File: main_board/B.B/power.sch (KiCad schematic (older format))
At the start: 30 parts, among them Q1 2N7002, Q2 2N7002, Q5 SI3447CDV, SW3 SW_DIP_x01, U62 SY8009, U63 FP6276

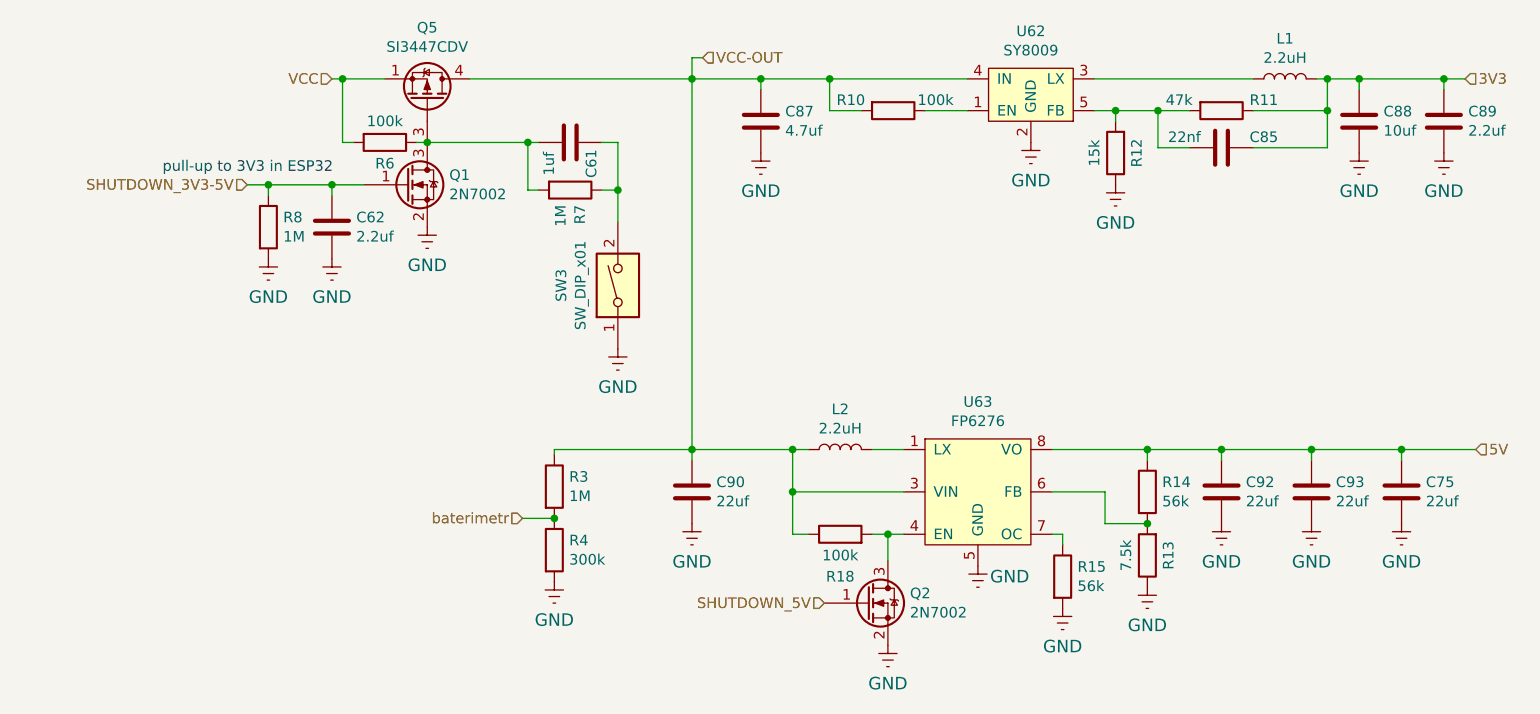
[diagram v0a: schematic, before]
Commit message: opravi_a_dodatky MPU/QMC/conn_A9G
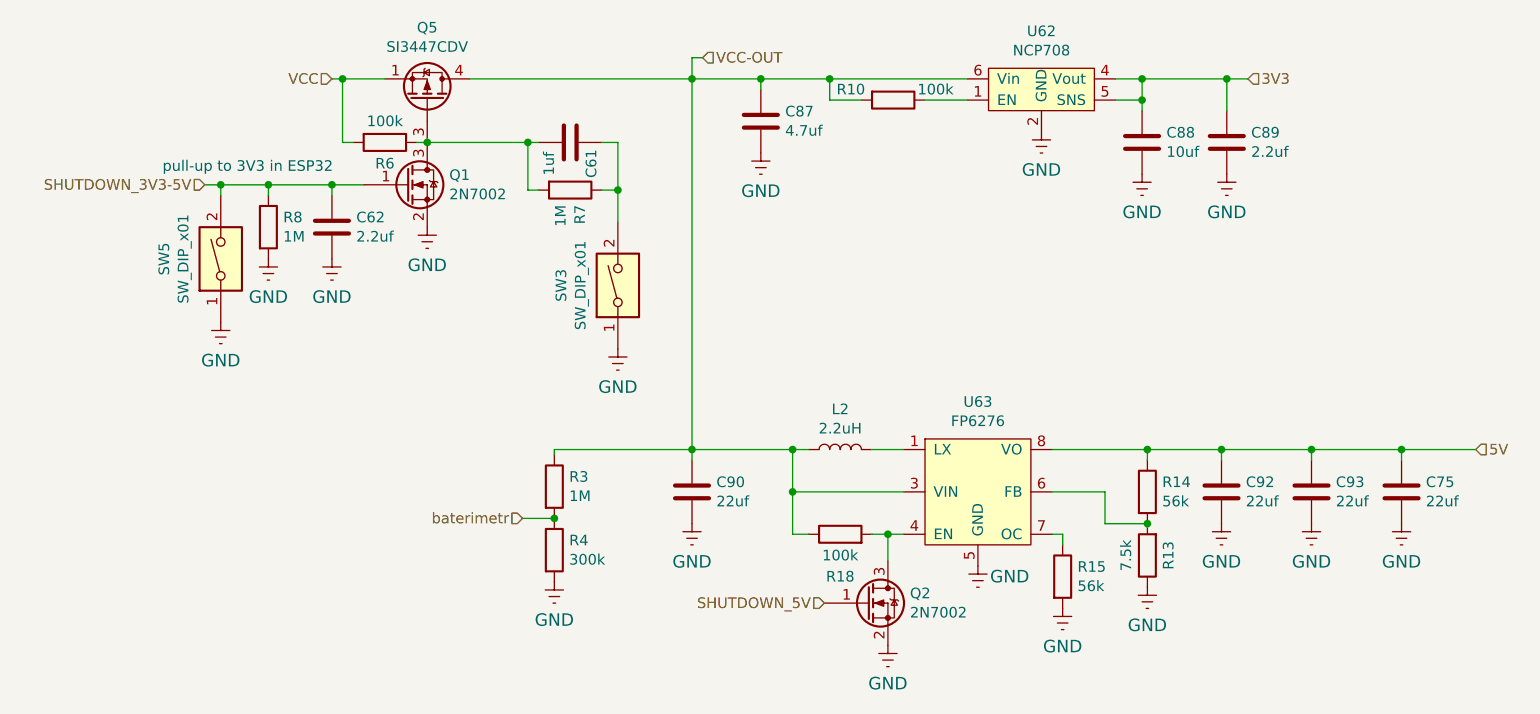
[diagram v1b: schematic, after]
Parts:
- removed C85: 22nf, Capacitor_SMD:C_0402_1005Metric, symbol B.B-rescue:C-Device-B.B-rescue
- removed L1: 2.2uH, BB:MWSA0603_6.6x7.1x3.0, symbol B.B-rescue:L-Device-B.B-rescue
- removed R11: 47k, Resistor_SMD:R_0402_1005Metric, symbol B.B-rescue:R-Device-B.B-rescue
- removed R12: 15k, Resistor_SMD:R_0402_1005Metric, symbol B.B-rescue:R-Device-B.B-rescue
- removed U62: SY8009, Package_TO_SOT_SMD:SOT-23-5, symbol B.B-rescue:SY8009
- added SW5: SW_DIP_x01, Button_Switch_SMD:SW_Push_1P1T_NO_CK_KSC6xxJ, symbol B.B-rescue:SW_DIP_x01-Switch-B.B-rescue
- added U62: NCP708, Package_DFN_QFN:DFN-6-1EP_3x3mm_P0.95mm_EP1.7x2.6mm, symbol B.B-rescue:NCP708
- U63: footprint Package_SO:SOP-8_3.76x4.96mm_P1.27mm -> Package_SO:SOIC-8-1EP_3.9x4.9mm_P1.27mm_EP2.41x3.81mm_ThermalVias
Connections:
- net 3V3: now also U62.4 (Vout), U62.5 (SNS)
- net SHUTDOWN_3V3-5V: now also SW5.2
- net VCC-OUT: now also U62.6 (Vin)
- net at R10.1: now also U62.1 (EN)
- new net GND: U62.2 (GND), U62.7 (GND)
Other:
- moved on the sheet: C88, C89, R10

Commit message: opravy_a_dodatky_2
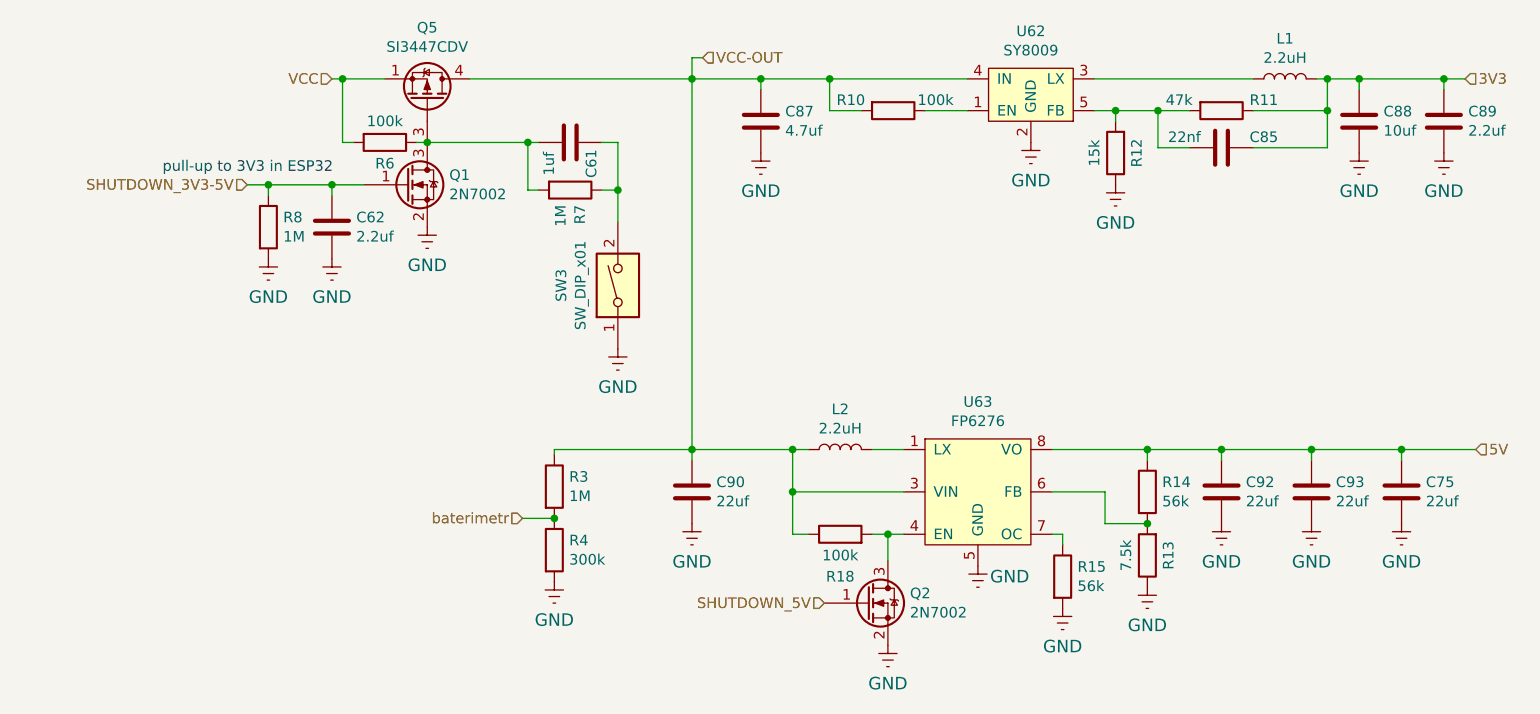
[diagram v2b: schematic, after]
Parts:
- removed SW5: SW_DIP_x01, Button_Switch_SMD:SW_Push_1P1T_NO_CK_KSC6xxJ, symbol B.B-rescue:SW_DIP_x01-Switch-B.B-rescue
- removed U62: NCP708, Package_DFN_QFN:DFN-6-1EP_3x3mm_P0.95mm_EP1.7x2.6mm, symbol B.B-rescue:NCP708
- added C85: 22nf, Capacitor_SMD:C_0402_1005Metric, symbol B.B-rescue:C-Device-B.B-rescue
- added L1: 2.2uH, BB:MWSA0603_6.6x7.1x3.0, symbol B.B-rescue:L-Device-B.B-rescue
- added R11: 47k, Resistor_SMD:R_0402_1005Metric, symbol B.B-rescue:R-Device-B.B-rescue
- added R12: 15k, Resistor_SMD:R_0402_1005Metric, symbol B.B-rescue:R-Device-B.B-rescue
- added U62: SY8009, Package_TO_SOT_SMD:SOT-23-5, symbol B.B-rescue:SY8009
- U63: footprint Package_SO:SOIC-8-1EP_3.9x4.9mm_P1.27mm_EP2.41x3.81mm_ThermalVias -> Package_SO:SOP-8_3.76x4.96mm_P1.27mm
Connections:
- net 3V3: now also C85.1, L1.2, R11.1
- net VCC-OUT: now also U62.4 (IN)
- net at R10.1: now also U62.1 (EN)
- new net: C85.2, R11.2, R12.2, U62.5 (FB)
- new net: L1.1, U62.3 (LX)
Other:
- moved on the sheet: C88, C89, R10
